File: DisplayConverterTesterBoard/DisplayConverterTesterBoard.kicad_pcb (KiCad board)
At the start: 2 copper layers, 24 parts, among them J2 Conn_01x07, J3 Conn_01x03, J4 FPC 20PIN P0.5mm, J5 BM20B(0.8)-10DS-0.4V, J6 Conn_01x03, J7 FPC 10PIN P0.5mm, U2 TPS61040DBV

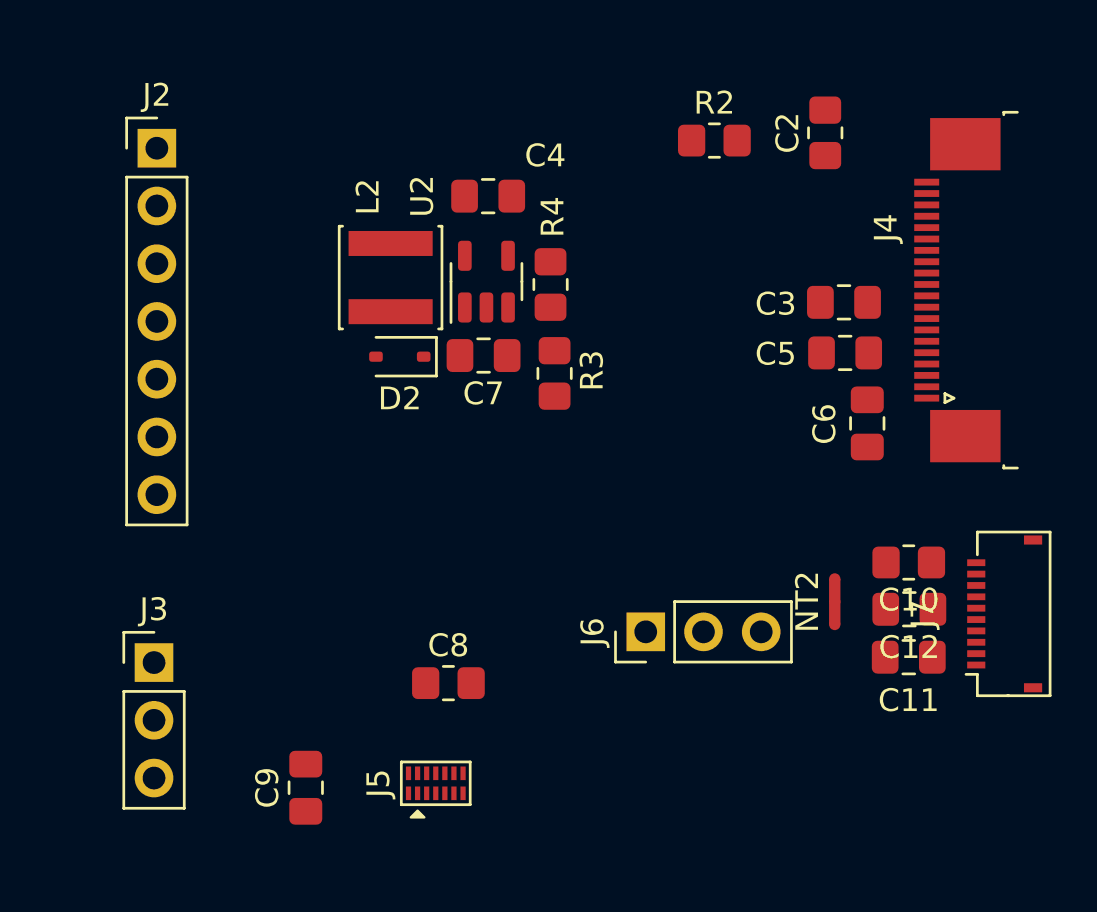
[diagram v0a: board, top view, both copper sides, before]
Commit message: routed
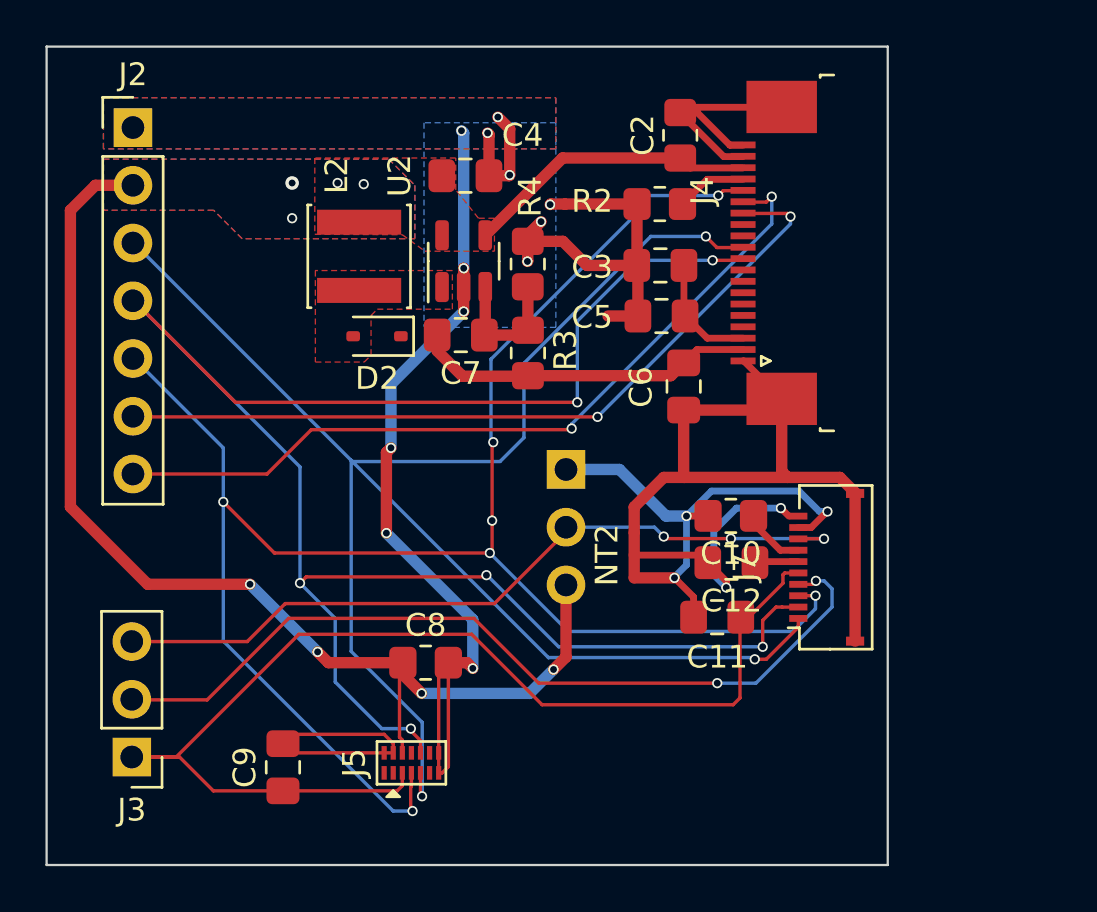
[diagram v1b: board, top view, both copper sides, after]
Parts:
- J6: moved to B.Cu
- moved NT2 9.06 mm to (112.3, 82.3)
- moved C11 8.61 mm to (115.9, 85.0)
- moved J4 8.24 mm to (118.4, 69.0)
- moved C3 8.24 mm to (113.4, 69.5)
- moved C5 8.24 mm to (113.5, 71.8)
- moved C6 8.24 mm to (114.5, 74.9)
- moved C12 8.09 mm to (116.6, 82.6)
- moved C10 8.09 mm to (116.5, 80.5)
- moved J7 8.09 mm to (120.9, 82.8)
- moved J6 7.96 mm to (109.3, 78.5), turned to 180 degrees
- moved C2 6.38 mm to (114.3, 63.8)
- moved J3 4.27 mm to (90.2, 91.2), turned to 180 degrees
- moved R2 3.68 mm to (113.4, 66.8), turned to 180 degrees
- moved L2 1.67 mm to (100.2, 69.1)
- moved R3 1.48 mm to (107.6, 73.4)
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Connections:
- net +3V3 renamed /3V3
- net Net-(D2-A) renamed /OLED 0.6"/SW
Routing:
- net GND: track 0.00 -> 114.7 mm, vias 0 -> 12
- net /MOSI: track 0.00 -> 84.0 mm, vias 0 -> 6
- net /~{CS}: track 0.00 -> 80.5 mm, vias 0 -> 7
- net /SCK: track 0.00 -> 78.3 mm, vias 0 -> 3
- net /3V3: track 0.00 -> 65.4 mm, vias 0 -> 8
- net /DISP: track 0.00 -> 50.7 mm
- net /EXTCOMMIN: track 0.00 -> 37.2 mm, vias 0 -> 2
- net /~{RES}: track 0.00 -> 35.3 mm, vias 0 -> 2
- net /Data/~{Cmd}: track 0.00 -> 34.9 mm, vias 0 -> 2
- net /EXTMODE: track 0.00 -> 34.0 mm, vias 0 -> 3
- net VSS: track 0.00 -> 22.5 mm, vias 0 -> 3
- net +12V: track 0.00 -> 15.1 mm
- net VSSA: track 0.00 -> 10.9 mm, vias 0 -> 2
- net Net-(U2-FB): track 0.00 -> 5.98 mm
- net /OLED 0.6"/V_{COMH}: track 0.00 -> 5.20 mm
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- added copper zone on B.Cu, net /3V3
- added copper zone on F.Cu, net /3V3
- added copper zone on F.Cu, net /OLED 0.6"/SW
- added copper zone on B.Cu, net GND
- added copper zone on F.Cu, net GND
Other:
- board outline added: 37 x 36 mm
